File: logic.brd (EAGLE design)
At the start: 37.4 x 32.5 mm, 9 parts, among them CON1 PINHEAD_1X10-2, CON2 PINHEAD_1X10-2, CON4 PINHEAD_1X02-2, CON5 PINHEAD_1X02-2, CON6 PINHEAD_1X02-2, CON7 PINHEAD_1X07-2

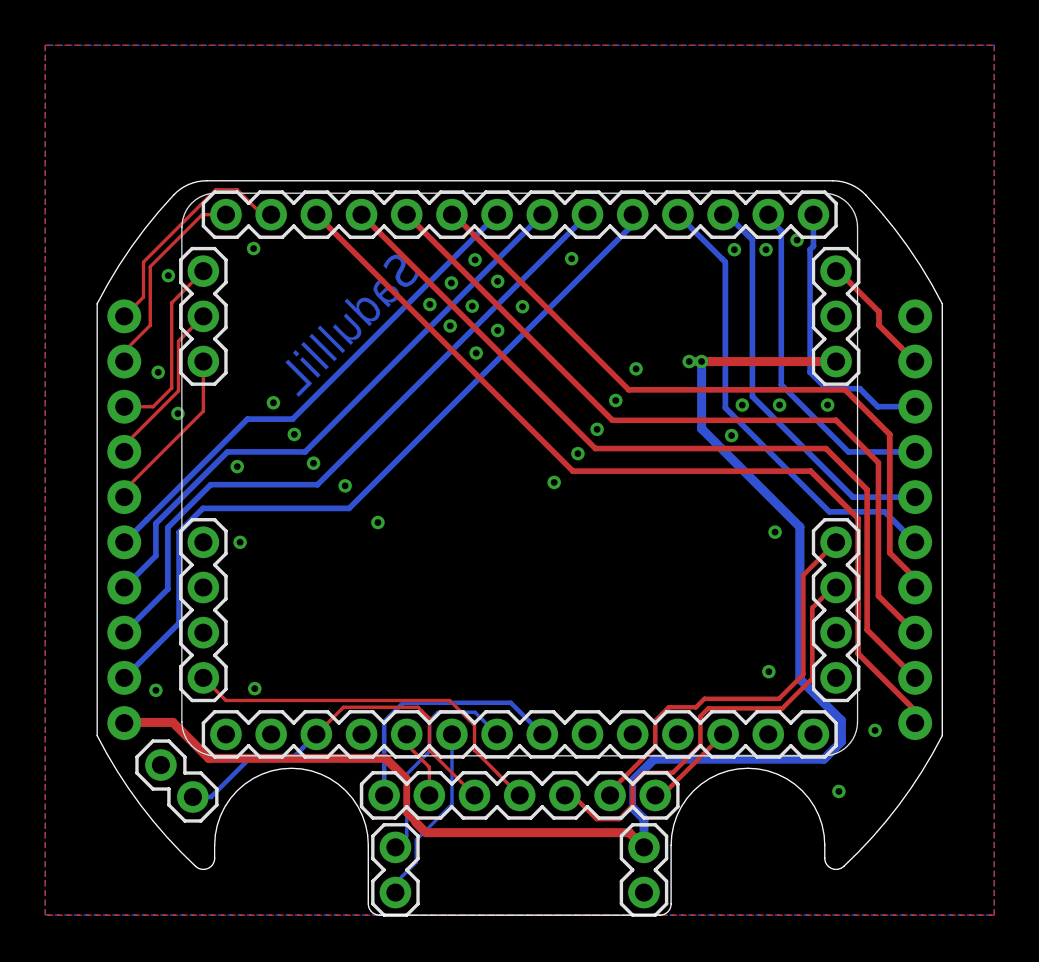
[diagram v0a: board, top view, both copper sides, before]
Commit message: bloody connectors
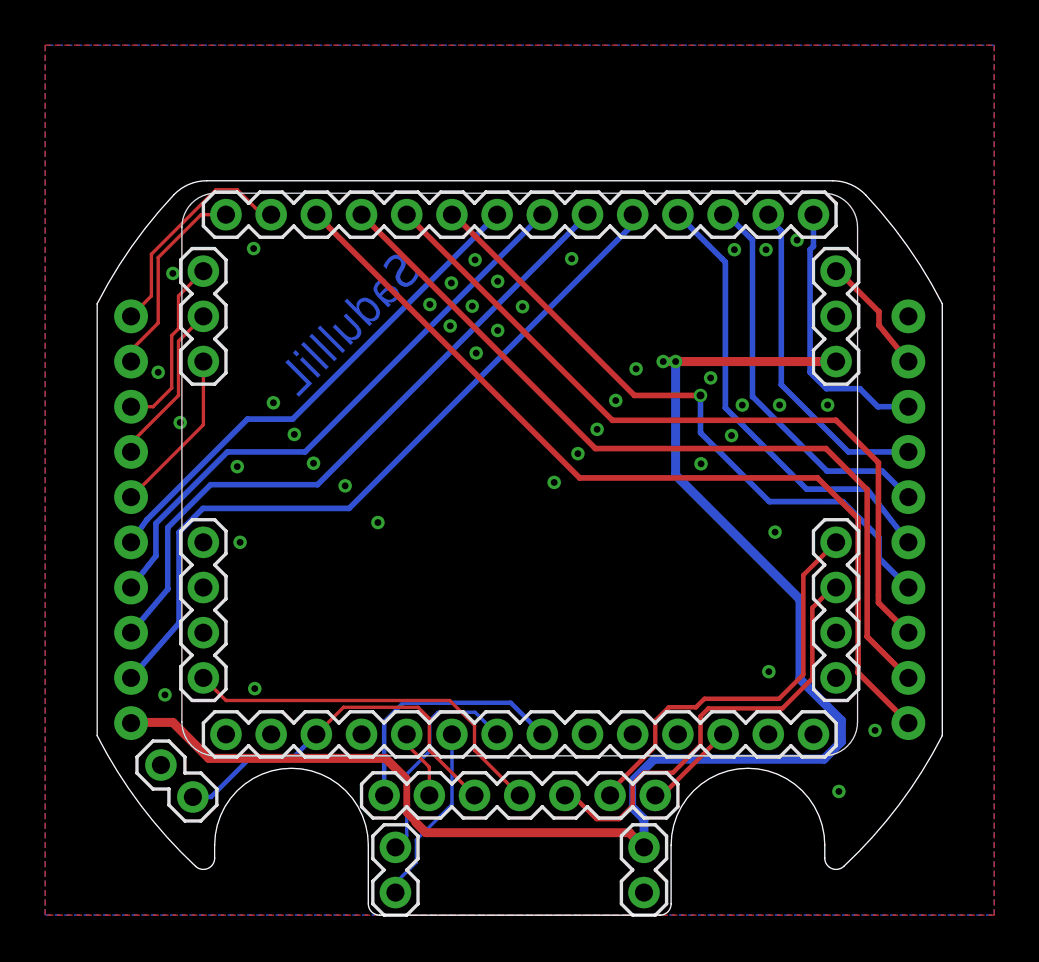
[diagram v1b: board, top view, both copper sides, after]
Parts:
- moved CON1 0.30 mm to (17.2, 0.00)
- moved CON2 0.30 mm to (-17.2, 0.00)
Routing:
- net PHASE_B_GATE_HIGH: track 30.6 -> 28.5 mm, vias 0 -> 1
- net VDD_5V: track 65.2 -> 67.0 mm
